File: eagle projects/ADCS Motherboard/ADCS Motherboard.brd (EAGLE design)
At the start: 91 x 91 mm, 140 parts, among them J1 HDR_10_EZFET_DEBUGGER, J11 CNC_3221-10-0300-00, J3 CNC_3221-10-0300-00, J5 CNC_3221-10-0300-00, J7 TE-1734829-3, J8 CNC_3221-10-0300-00, J9 CNC_3221-14-0300-00, Q1 PMV16XN, Q2 IRLML6246TRPBF, Q3 IRLML2246TRPBF, U1 MSP430F5529IPN, U2 LMV321, U3 ADS7841E_2K5, U4 LMV321, U5 LMV321, U7 HMC1053, Y1 32.768kHz, Y2 CSTCR4M00G15L99, Y3 32.768kHz

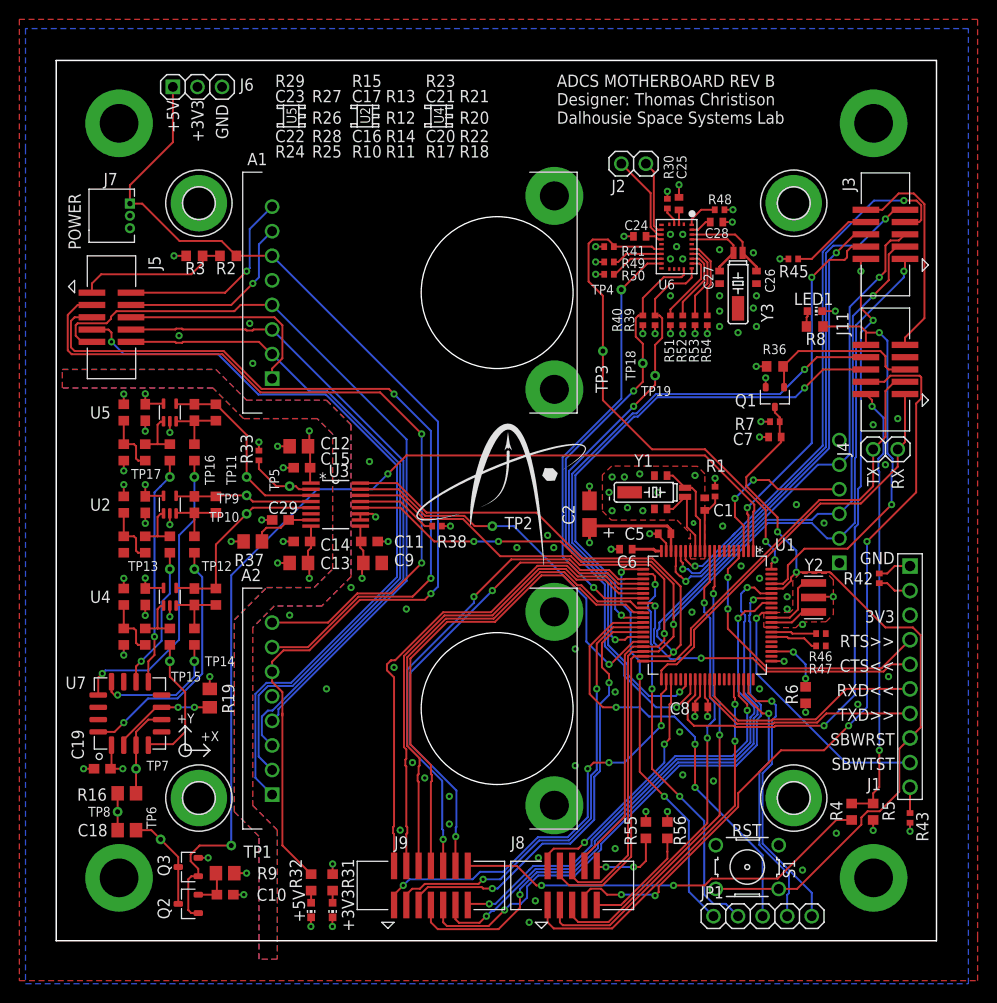
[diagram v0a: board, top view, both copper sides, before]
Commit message: Last commit before major layout changes on Actuator board Rev B
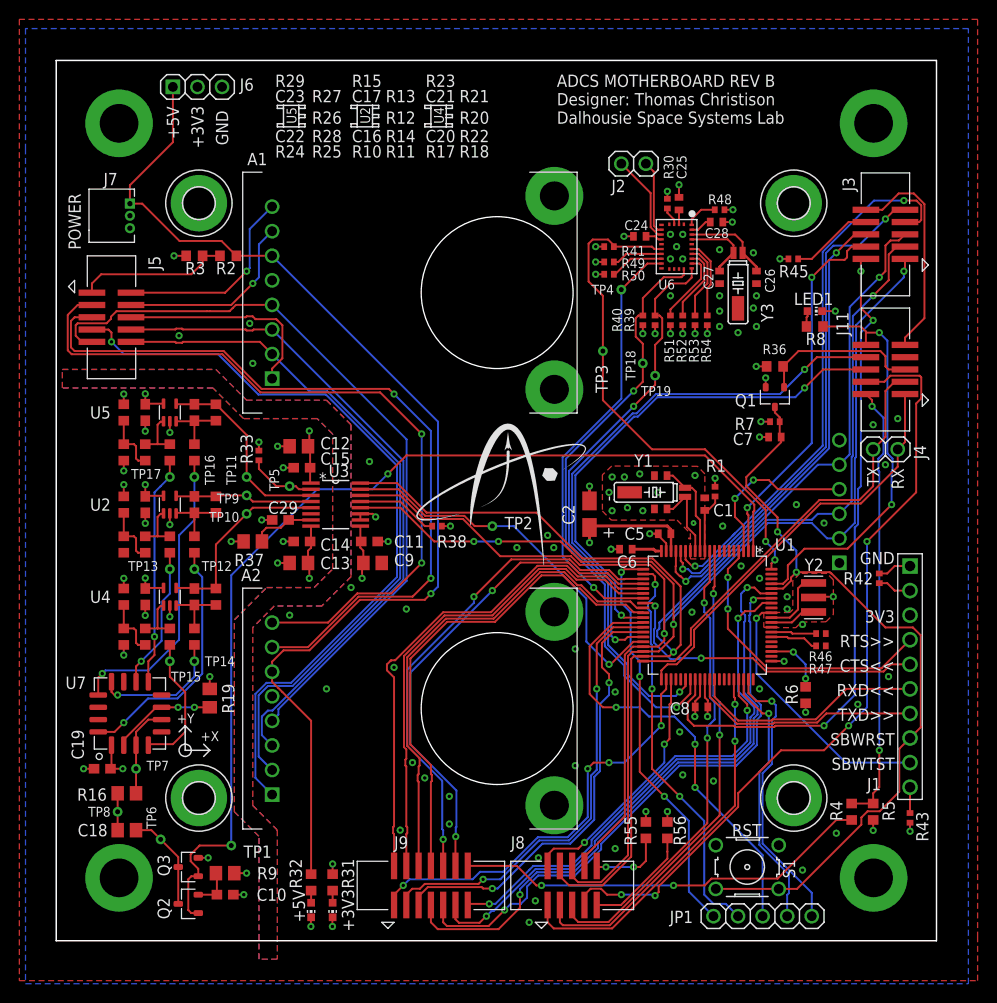
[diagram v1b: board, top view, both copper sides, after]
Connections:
- net !CS!_CURRENT_SENSE_1 renamed !CS!_CURR_SENSE_RW
- net !CS!_CURRENT_SENSE_2 renamed !CS!_CURR_SENSE_MTQR
